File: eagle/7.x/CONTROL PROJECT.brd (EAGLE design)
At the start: 107.9 x 67 mm, 27 parts, among them IC1 MEGA32-P

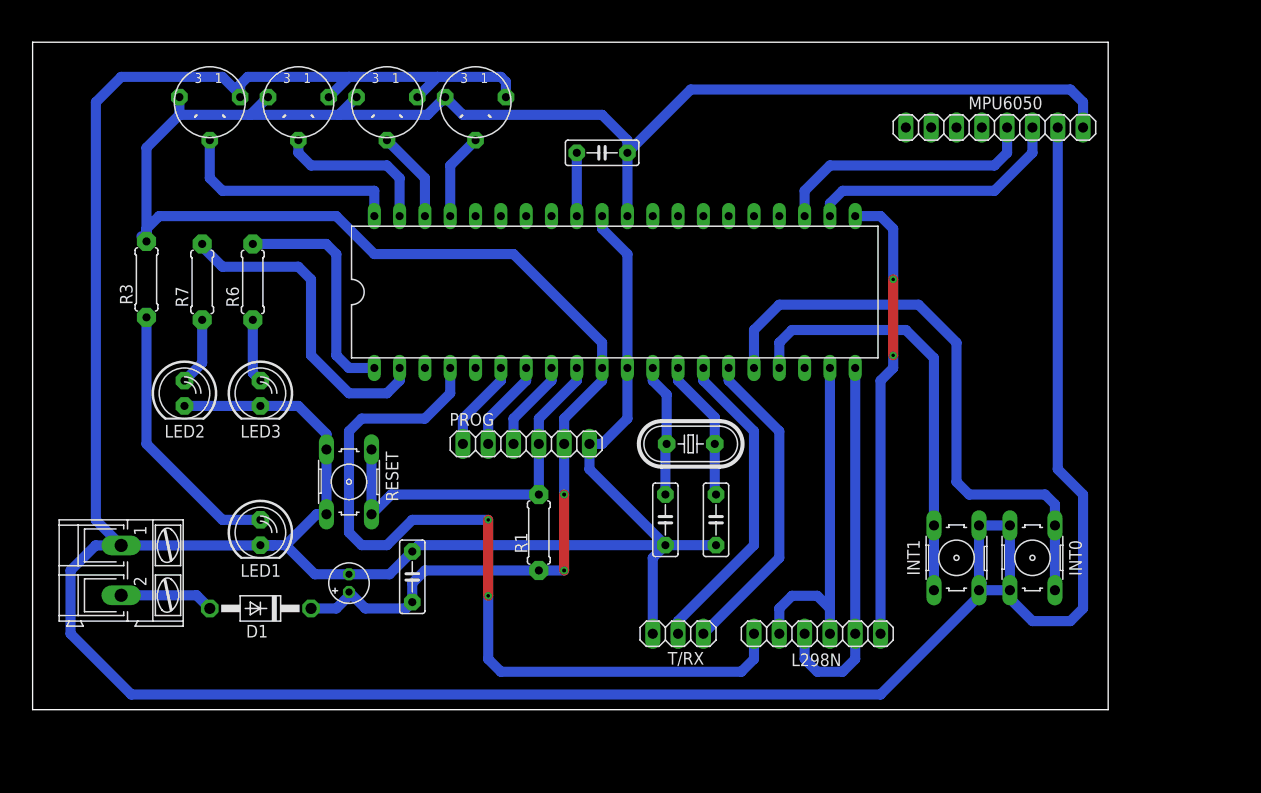
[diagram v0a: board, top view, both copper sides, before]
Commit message: v7
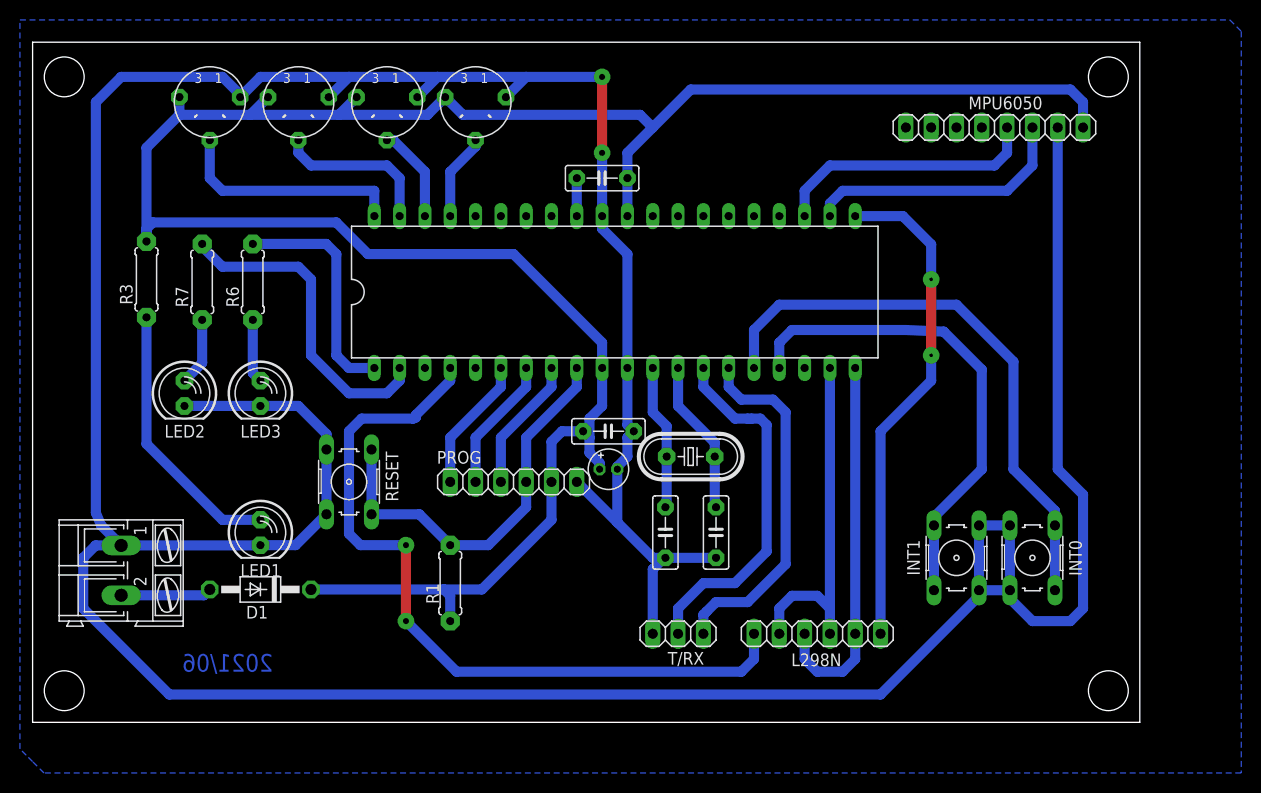
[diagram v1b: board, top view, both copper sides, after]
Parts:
- moved C4 28.4 mm to (61.6, 20.3), turned to 0 degrees
- moved C5 24.5 mm to (61.6, 24.1), turned to 180 degrees
- moved R1 10.2 mm to (45.7, 8.89)
- moved PROG 4.02 mm to (52.1, 19.1)
- moved C6 2.54 mm to (61.0, 49.5)
- moved D1 1.91 mm to (26.7, 8.26)
- moved C2 1.27 mm to (67.3, 14.0)
- moved C3 1.27 mm to (72.4, 14.0)
- moved Q1 1.27 mm to (69.8, 21.6)
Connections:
- net N$1 renamed SCL
- net N$13 renamed SDA
- net N$18 renamed SCK
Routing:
- net GND: track 427.8 -> 410.7 mm, vias 0 -> 2
- net OC0: track 84.2 -> 77.8 mm
- net IN1: track 43.0 -> 49.1 mm
- net OC2: track 45.5 -> 50.0 mm
- net RX: track 31.9 -> 36.3 mm
- net SCK: track 9.20 -> 13.5 mm
- net MOSI: track 9.20 -> 13.5 mm
- net MISO: track 9.20 -> 13.5 mm
- net TX: track 31.9 -> 36.2 mm
- net RESET: track 38.4 -> 41.0 mm
- net AREF: track 6.35 -> 3.81 mm
- net IN0: track 60.2 -> 57.9 mm
- net VCC: track 235.0 -> 236.8 mm, vias 2 -> 0
- net N$2: track 13.3 -> 14.6 mm
- net N$3: track 14.3 -> 15.5 mm
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- added copper zone on layer 16, net GND
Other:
- board size 107.9 x 67 mm -> 111.1 x 68.2 mm
- board text added: "2021/06"
